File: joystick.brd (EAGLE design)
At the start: 38.1 x 38.1 mm, 3 parts, among them U1 JOYSTICKPTH

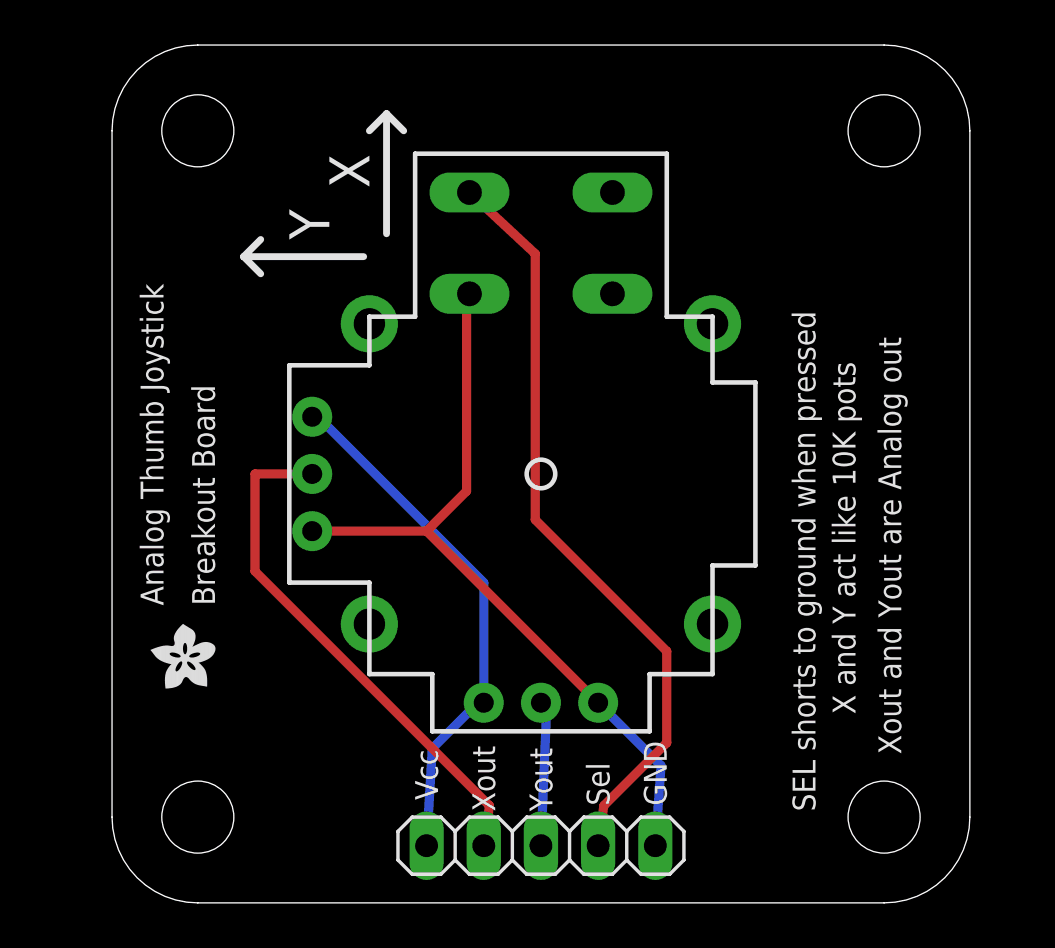
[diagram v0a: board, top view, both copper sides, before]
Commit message: Initial upload of fork
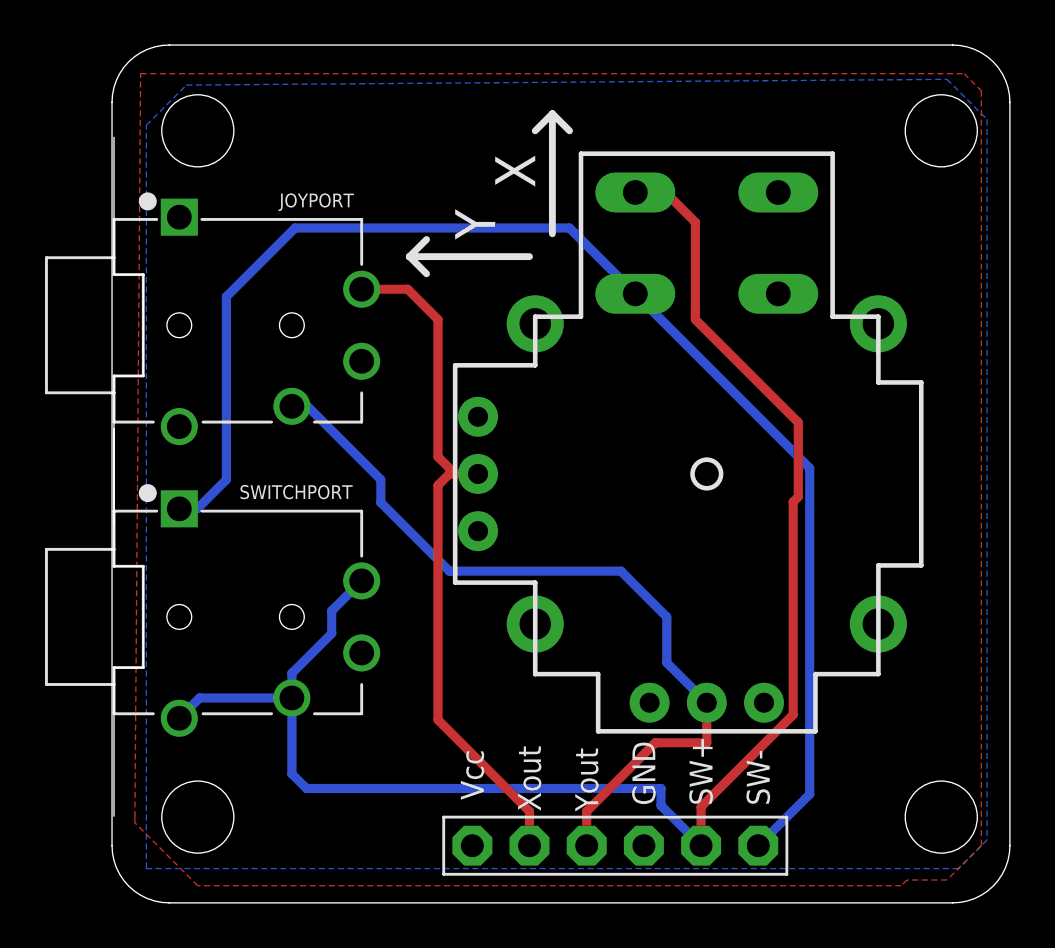
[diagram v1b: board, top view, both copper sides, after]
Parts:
- removed U$1: (no value), adafruit:ADAFRUIT200MIL
- added JOYPORT, SWITCHPORT: SJ-43515TS, ATMakers:CUI_SJ-43515TS
- JP1: device pinhead:1X05 -> adafruit:1X06-BIG
- moved U1 7.37 mm to (26.4, 19.1)
- moved JP1 3.30 mm to (22.4, 2.54)
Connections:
- removed net N$1: JP1.5, U1.H1, U1.V1
- new net GND: JOYPORT.4, JP1.3, U1.H3, U1.V3
- new net VCC: JOYPORT.1, JP1.6, U1.H1, U1.V1
- net N$2: now also JP1.2, SWITCHPORT.2, SWITCHPORT.3, SWITCHPORT.4, U1.B1A; no longer JP1.1, U1.B2A, U1.H3, U1.V3
- net N$3: now also JOYPORT.3, JP1.5; no longer JP1.4
- net N$4: now also JOYPORT.2, JP1.4; no longer JP1.3
- net N$5: now also JP1.1, SWITCHPORT.1, U1.B2A; no longer JP1.2, U1.B1A
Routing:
- net N$2: track 34.7 -> 71.5 mm
- net N$4: track 6.46 -> 35.6 mm
- net N$5: track 33.9 -> 60.1 mm
- net N$1: track 23.5 -> 0.00 mm
- net N$3: track 23.4 -> 31.8 mm
- added copper zone on layer 16, net GND
- added copper zone on layer 1, net VCC
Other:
- board size 38.1 x 38.1 mm -> 39.9 x 38.1 mm
- board text added: "#_______________"
- board text added: "ATMakers"
- board text added: "Rev A"
- board text added: "SW+"
- board text added: "SW-"
- board text added: "Thumb Stick"
- board text removed: "Analog Thumb Joystick"
- board text removed: "Breakout Board"
- board text removed: "SEL shorts to ground when pressed"
- board text removed: "Sel"
- board text removed: "X and Y act like 10K pots"
- board text removed: "Xout and Yout are Analog out"
